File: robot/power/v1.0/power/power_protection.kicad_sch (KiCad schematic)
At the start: 29 parts, among them Q1 BSC070N10NS5, Q2 BSC070N10NS5, Q3 2N7002, Q4 MMBT5401LT1G, SW1 HDR_2P, SW2 CPG151101D91, U3 LTC2955-2

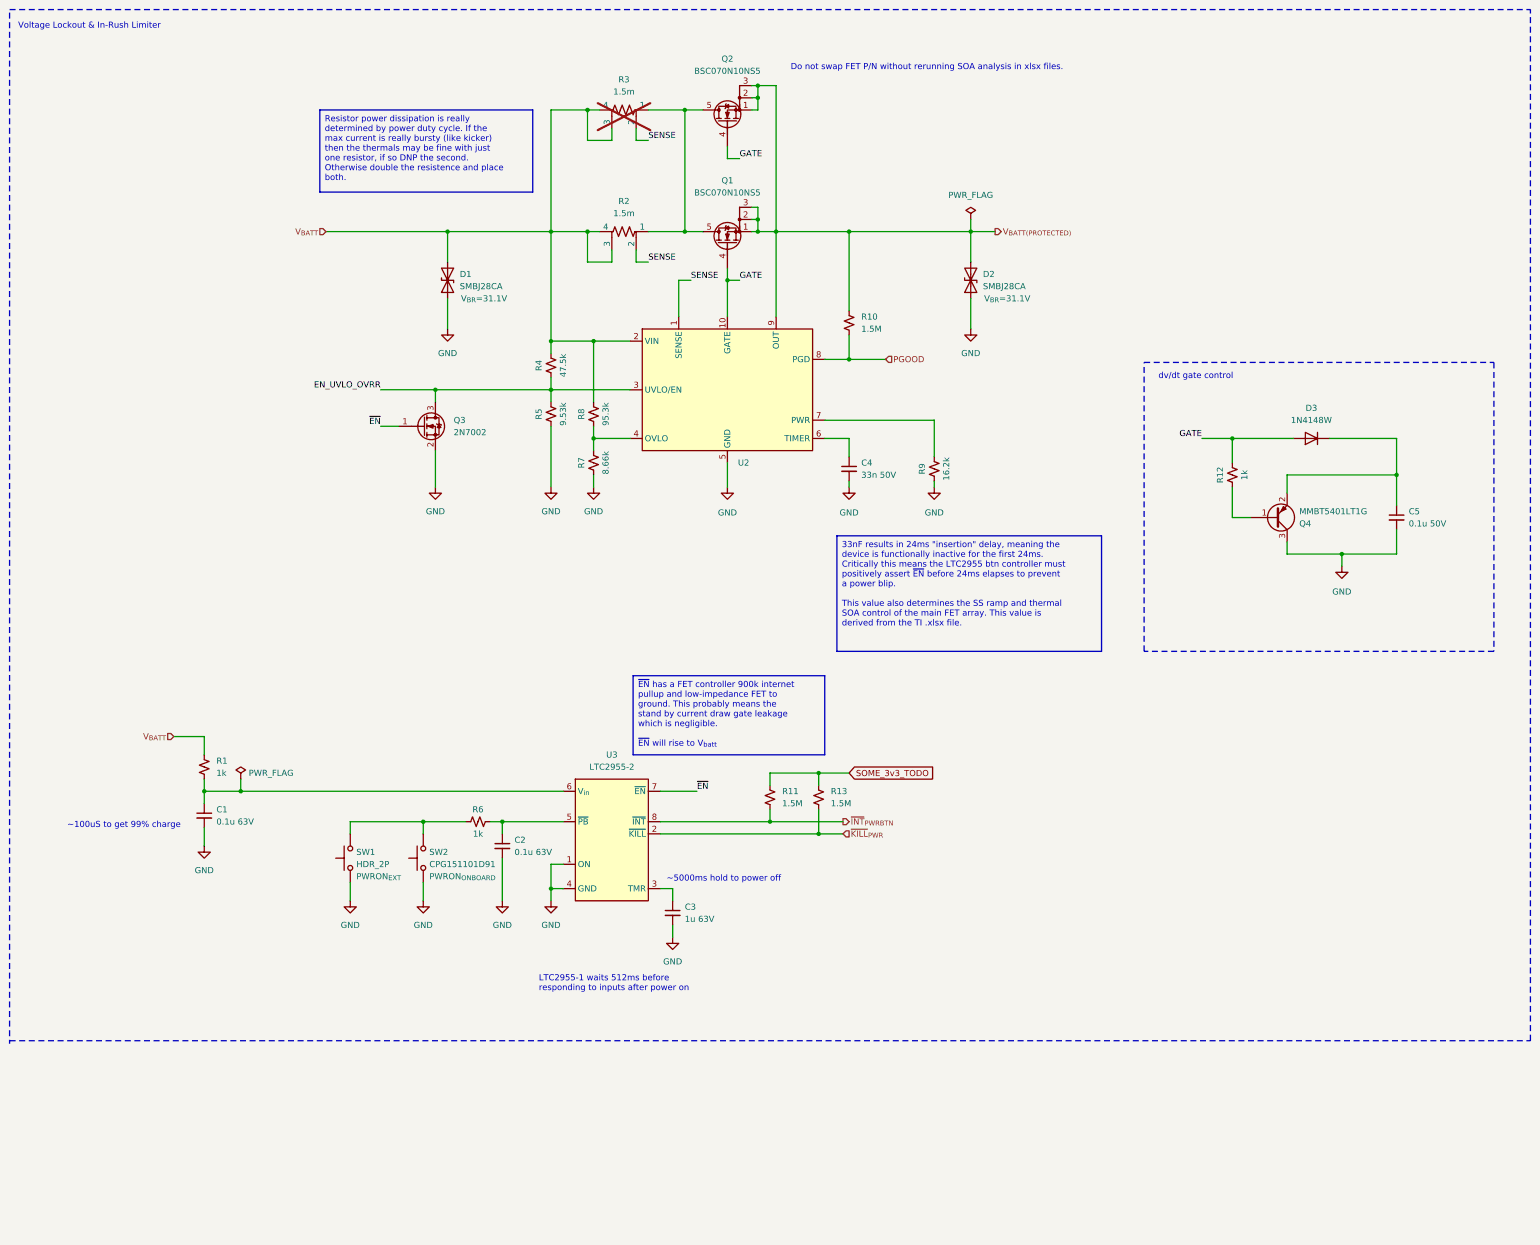
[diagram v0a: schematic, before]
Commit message: power schematic work
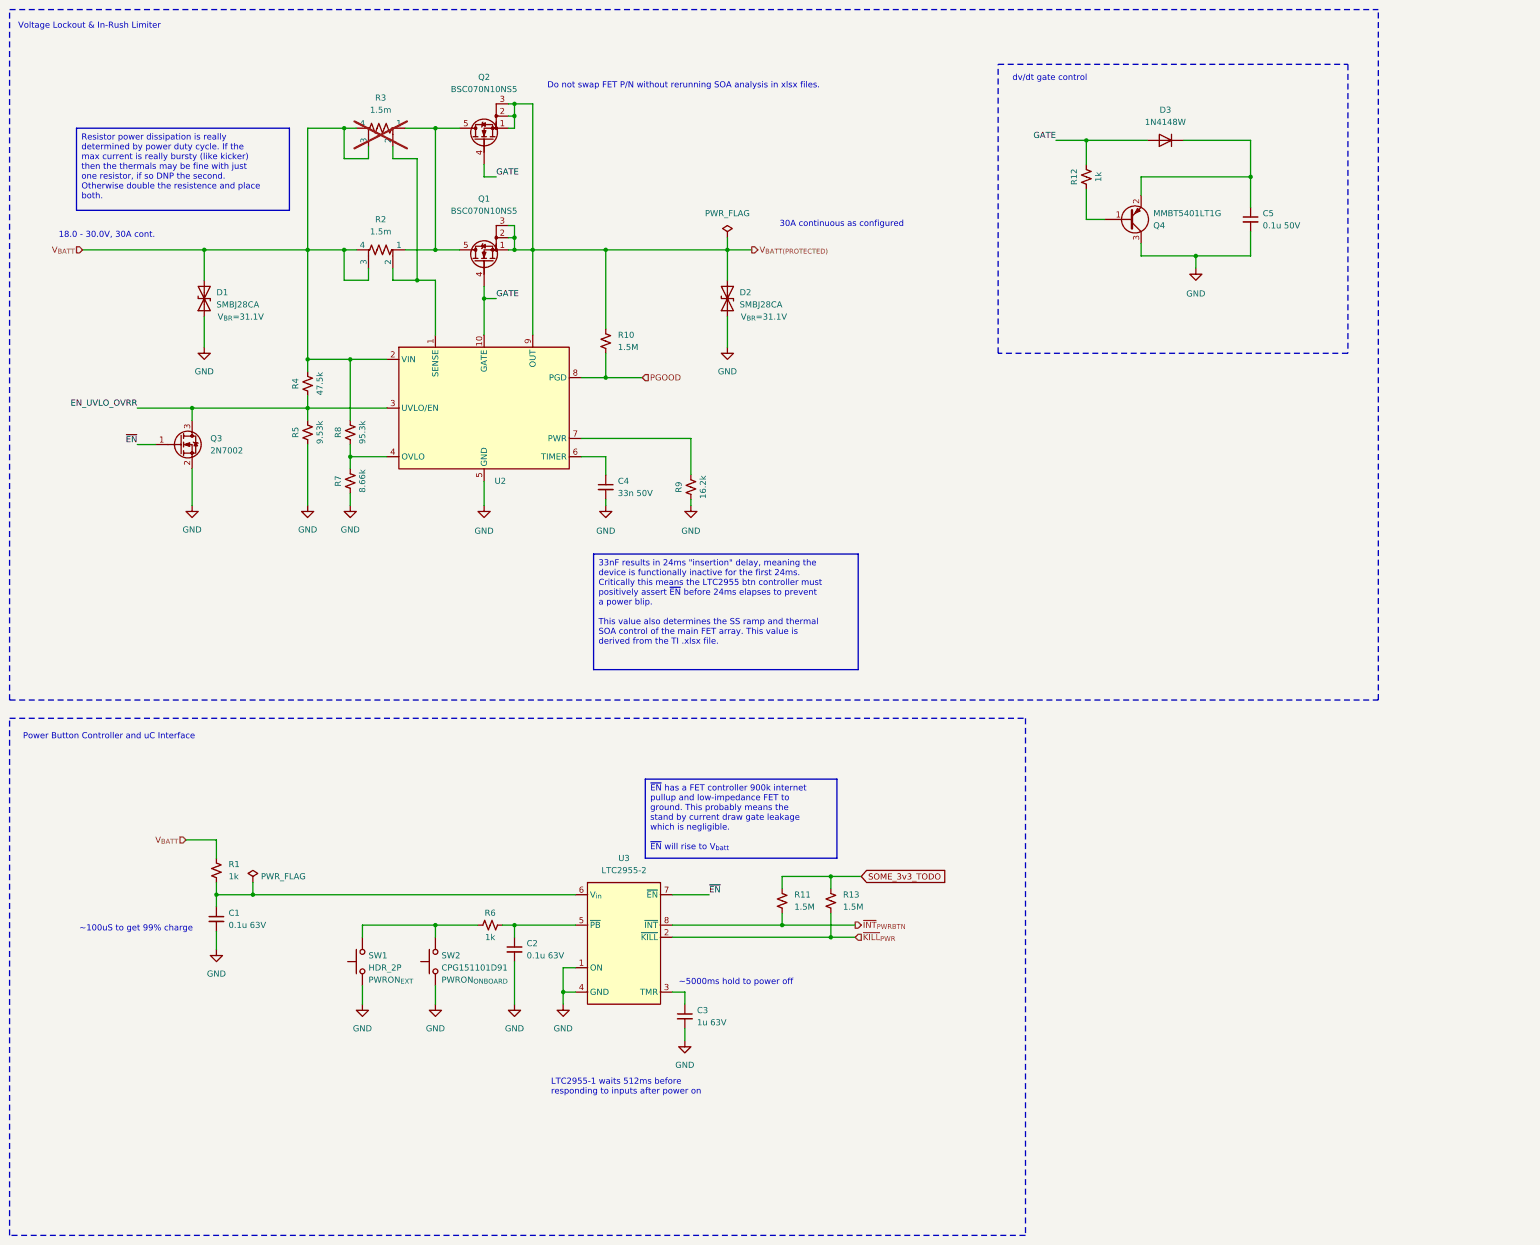
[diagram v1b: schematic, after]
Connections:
- net SENSE: no longer names the net of R2.2, R3.2, U2.1 (SENSE)
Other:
- note added: "18.0 - 30.0V, 30A cont."
- note added: "30A continuous as configured"
- note added: "Power Button Controller and uC Interface"
- moved on the sheet: C1, C2, C3, C4, C5, D1, D2, D3, Q1, Q2, Q3, Q4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
